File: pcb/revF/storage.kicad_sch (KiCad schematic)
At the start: 18 parts, among them CON1 CF CARD, CON2 SD CARD, CON9 uSD CARD, Q1 BC856

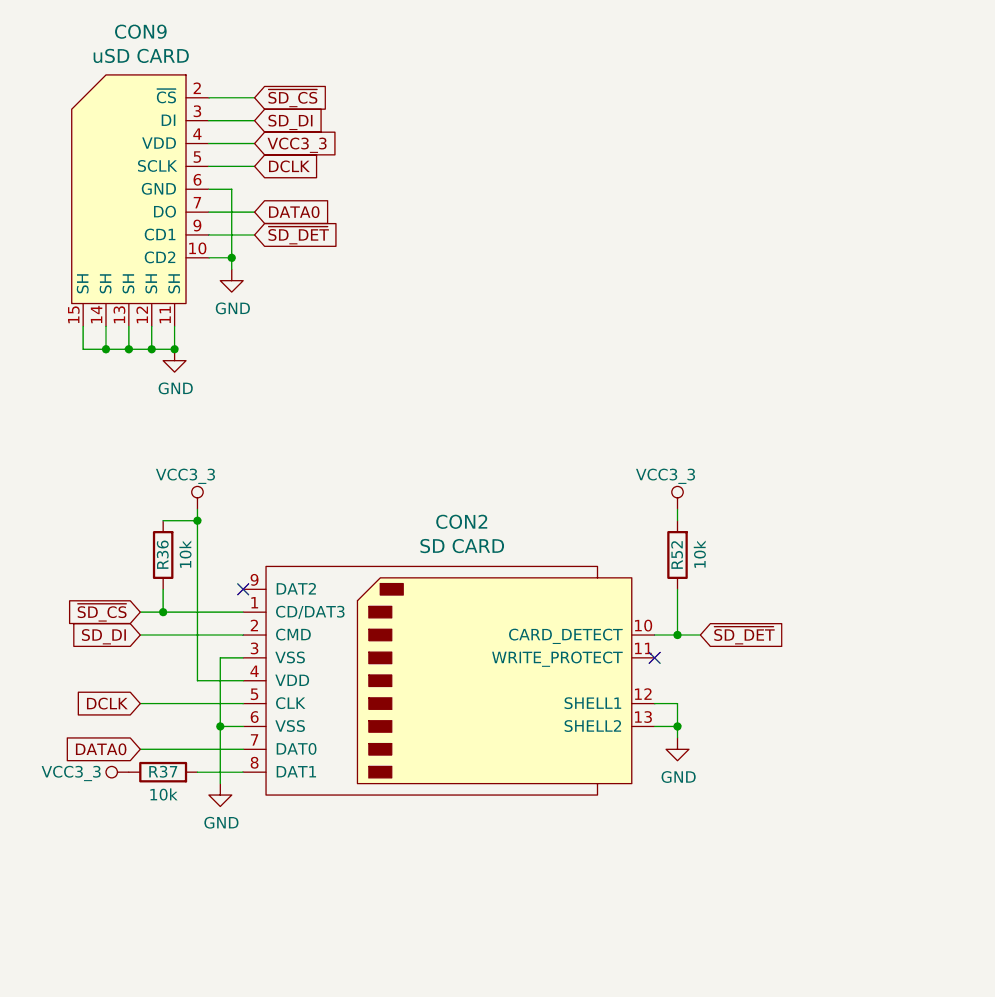
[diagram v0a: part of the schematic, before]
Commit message: New schematics / revF
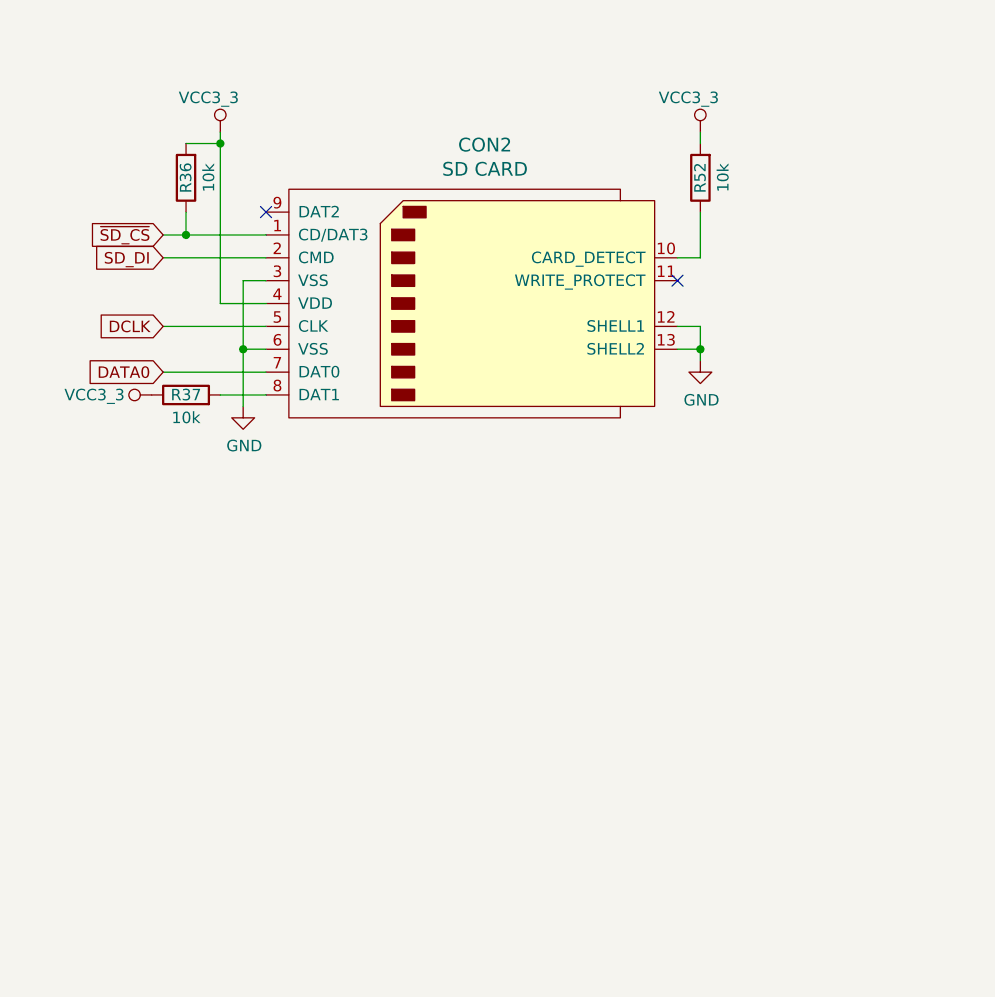
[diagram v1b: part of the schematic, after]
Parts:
- removed CON9: uSD CARD, footprints:Conn_uSDcard, symbol retro:MicroSD_Molex
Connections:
- net ~{SD_DET}: no longer names the net of CON2.10 (CARD_DETECT), R52.1
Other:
- moved on the sheet: CON2, R36, R37, R52
